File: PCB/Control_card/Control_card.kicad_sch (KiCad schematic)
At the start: 46 parts, among them IC1 TLSR8253F512ET48, J1 Conn_02x04_Counter_Clockwise, J2 Conn_01x01_Pin, J3 Conn_01x01_Pin, J4 Conn_01x01_Pin, J5 Conn_01x01_Pin, Y1 Crystal_GND24

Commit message: Ajout des footprints
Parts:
- J1: footprint Touch_Switch_Custom:Pin mâle -> Touch_Switch_Custom:PinMale
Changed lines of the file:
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@@
 			)
 		)
-		(property "Footprint" "Touch_Switch_Custom:Pin mâle"
+		(property "Footprint" "Touch_Switch_Custom:PinMale"
 			(at 39.37 29.21 0)
 			(effects

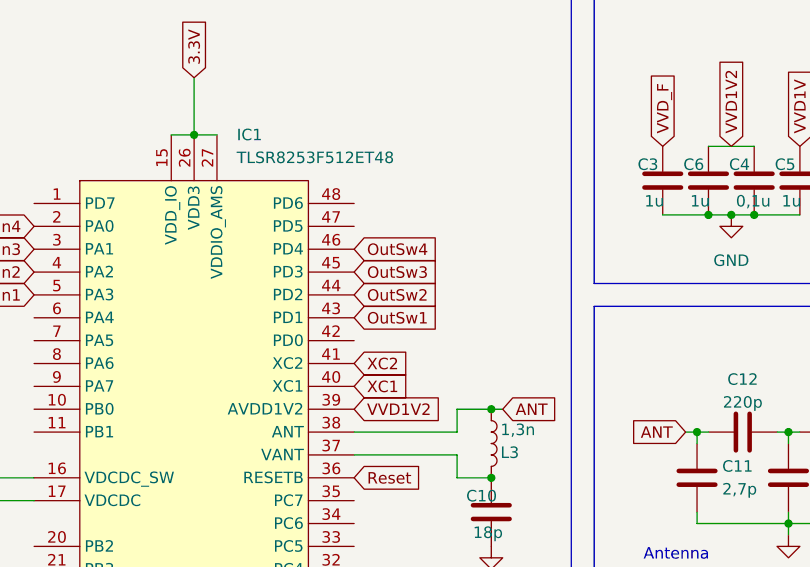
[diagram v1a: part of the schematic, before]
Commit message: Rota IC contrôle
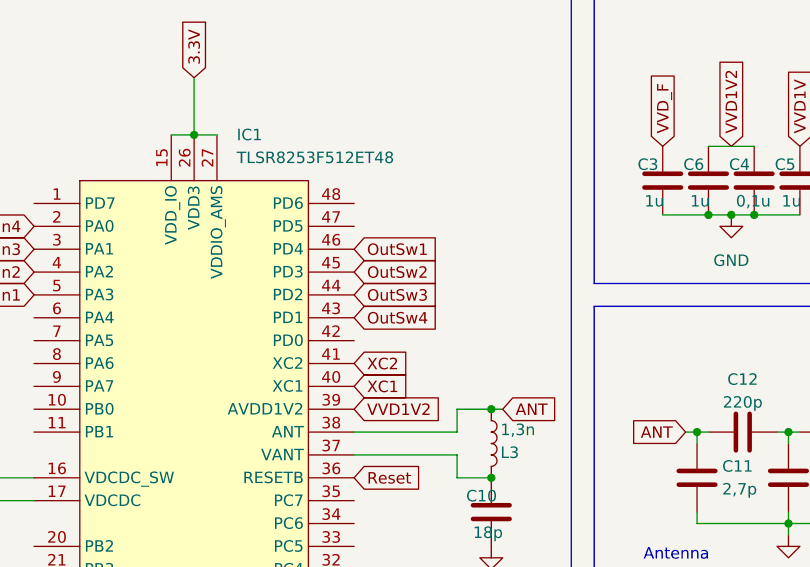
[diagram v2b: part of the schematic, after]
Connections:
- net OutSw1: now also IC1.46 (PD4); no longer IC1.43 (PD1)
- net OutSw2: now also IC1.45 (PD3); no longer IC1.44 (PD2)
- net OutSw3: now also IC1.44 (PD2); no longer IC1.45 (PD3)
- net OutSw4: now also IC1.43 (PD1); no longer IC1.46 (PD4)
